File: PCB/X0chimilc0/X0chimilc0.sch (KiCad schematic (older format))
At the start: 0 parts

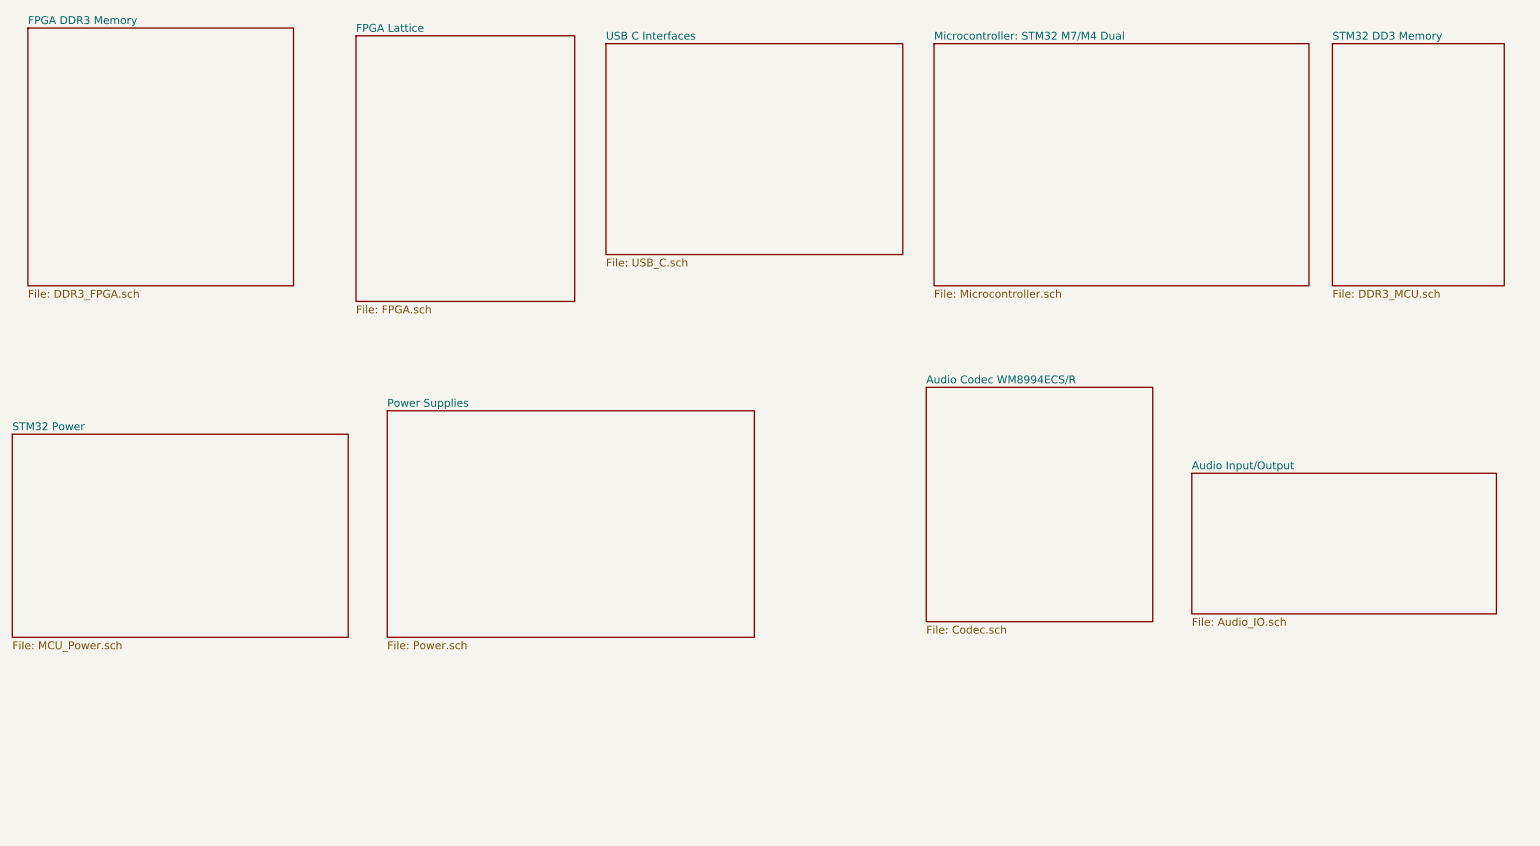
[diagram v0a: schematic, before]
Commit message: USB C DDR3L MCU
more with MCU and USB C and DDR3L
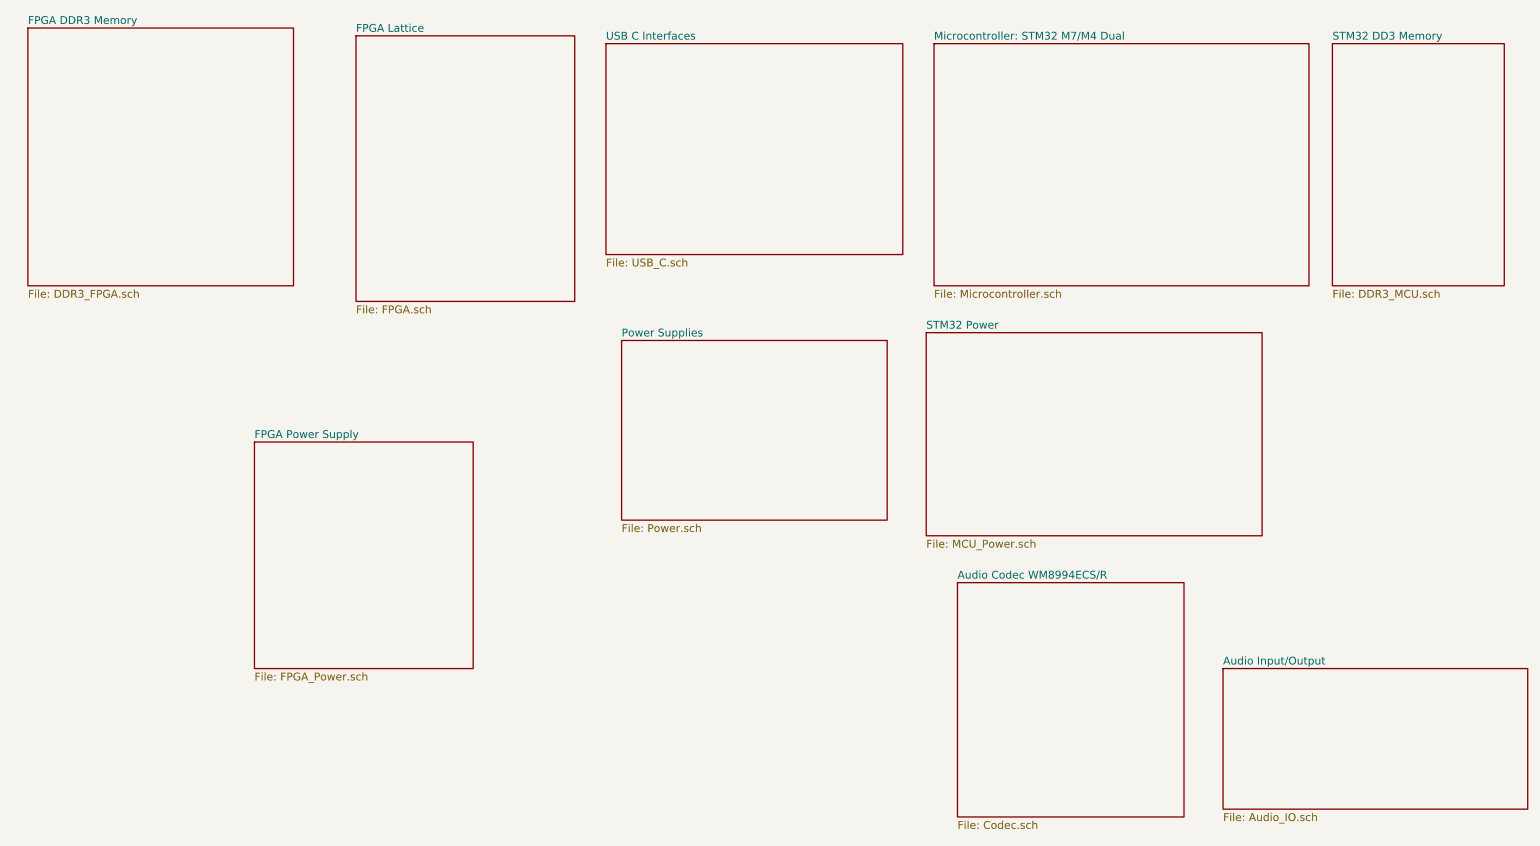
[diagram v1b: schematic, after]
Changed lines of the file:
@@
 $Descr A4 11693 8268
 encoding utf-8
-Sheet 1 10
+Sheet 1 11
 Title ""
 Date ""
@@
 Comment4 ""
 $EndDescr
-$Sheet
-S 3400 3600 2350 1450
-U 5E2ACA94
-F0 "Power Supplies" 50
-F1 "Power.sch" 50
-$EndSheet
 $Sheet
 S 6900 1250 2400 1550
@@
 $EndSheet
 $Sheet
-S 6850 3450 1450 1500
+S 7050 4700 1450 1500
 U 5E30BDF7
 F0 "Audio Codec WM8994ECS/R" 50
@@
 $EndSheet
 $Sheet
-S 1000 3750 2150 1300
+S 6850 3100 2150 1300
 U 5E02C3CE
 F0 "STM32 Power " 50
@@
 $EndSheet
 $Sheet
-S 8550 4000 1950 900
+S 8750 5250 1950 900
 U 5E1A79E6
 F0 "Audio Input/Output" 50
@@
 F1 "USB_C.sch" 50
 $EndSheet
+$Sheet
+S 2550 3800 1400 1450
+U 5EA384BF
+F0 "FPGA Power Supply" 50
+F1 "FPGA_Power.sch" 50
+$EndSheet
+$Sheet
+S 4900 3150 1700 1150
+U 5E2ACA94
+F0 "Power Supplies" 50
+F1 "Power.sch" 50
+$EndSheet
 $EndSCHEMATC
